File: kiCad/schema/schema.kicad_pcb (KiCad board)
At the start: 2 copper layers, 90 x 127.1 mm, 30 parts, among them J1 Conn_01x06_Pin, J11 Switch, J14 Conn_01x06_Pin, J15 MOSFET, J2 Esp32, J3 M1 Right, J4 M2 Left, J5 Bat, J6 Buck, Q1 Q_Photo_NPN, Q2 Q_Photo_NPN, Q3 Q_Photo_NPN, Q4 Q_Photo_NPN

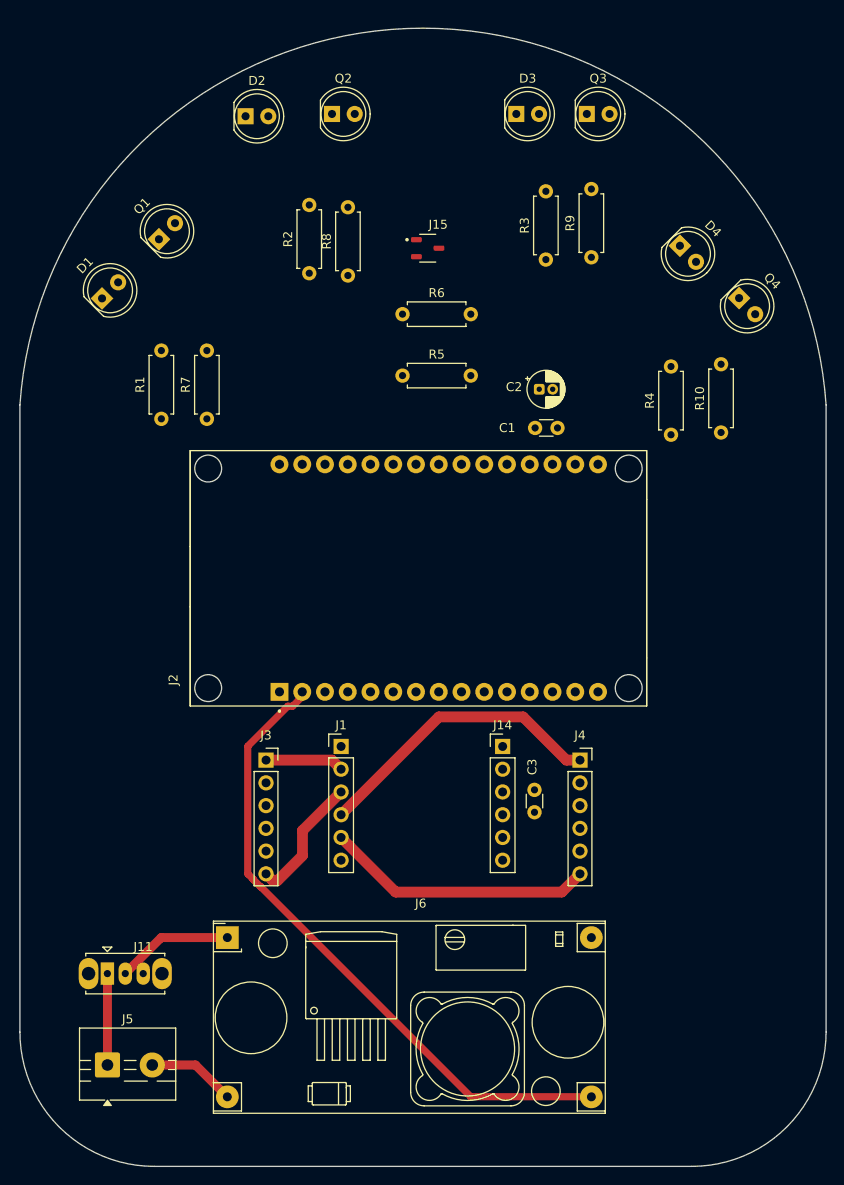
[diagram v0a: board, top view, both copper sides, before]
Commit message: Day 17 - PCB 60% Done
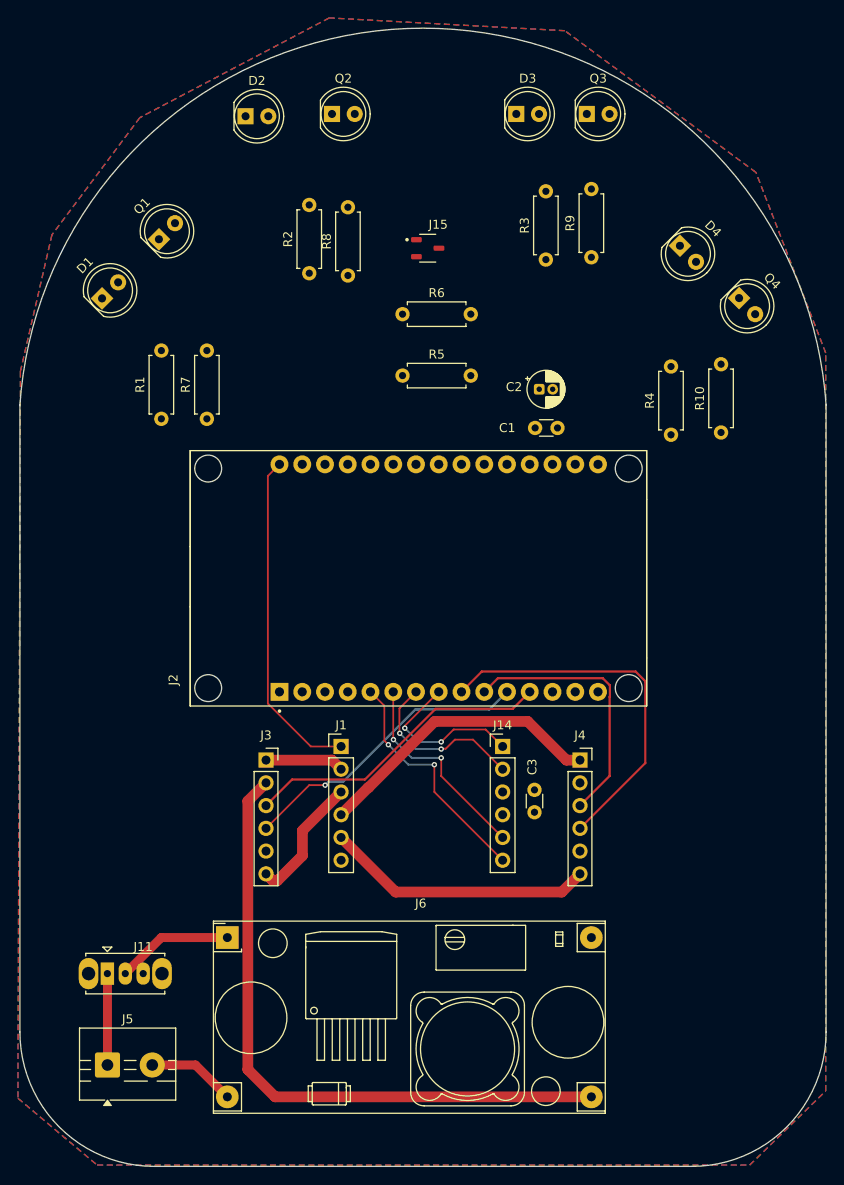
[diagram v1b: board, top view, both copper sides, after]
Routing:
- net /ENC B2: track 0.00 -> 41.4 mm
- net /3V3: track 0.00 -> 37.4 mm
- net /ENC A1: track 0.00 -> 34.7 mm
- net /ENC A2: track 0.00 -> 33.2 mm, vias 0 -> 1
- net /ENC B1: track 0.00 -> 29.8 mm
- net /BIN 2: track 0.00 -> 26.6 mm, vias 0 -> 2
- net /BIN 1: track 0.00 -> 23.2 mm, vias 0 -> 2
- net /AIN 2: track 0.00 -> 19.5 mm, vias 0 -> 2
- net /AIN 1: track 0.00 -> 18.6 mm, vias 0 -> 2
- net /BUCK +: track 71.8 -> 73.0 mm
- added copper zone on B.Cu, net /GND
- added copper zone on F.Cu, net /GND
